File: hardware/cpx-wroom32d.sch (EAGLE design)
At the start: 37 parts, among them Q1 mmbt2222, Q2 mmbt2222, U1 ESP32-WROOM-32D

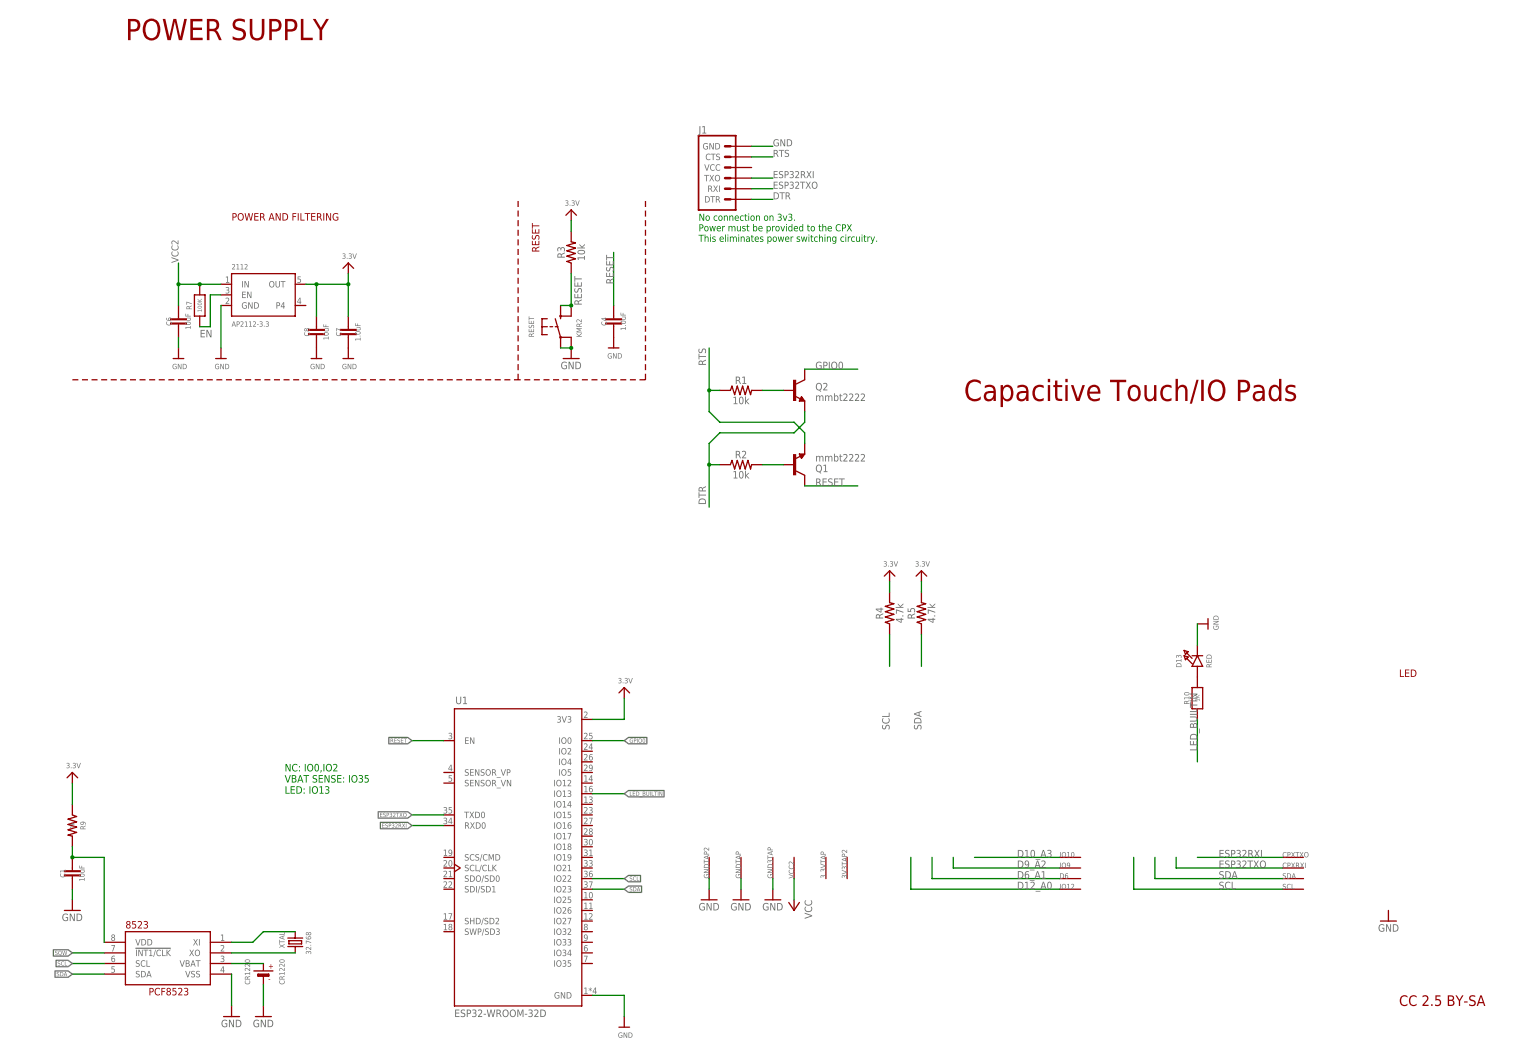
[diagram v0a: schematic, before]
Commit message: Looks goo.
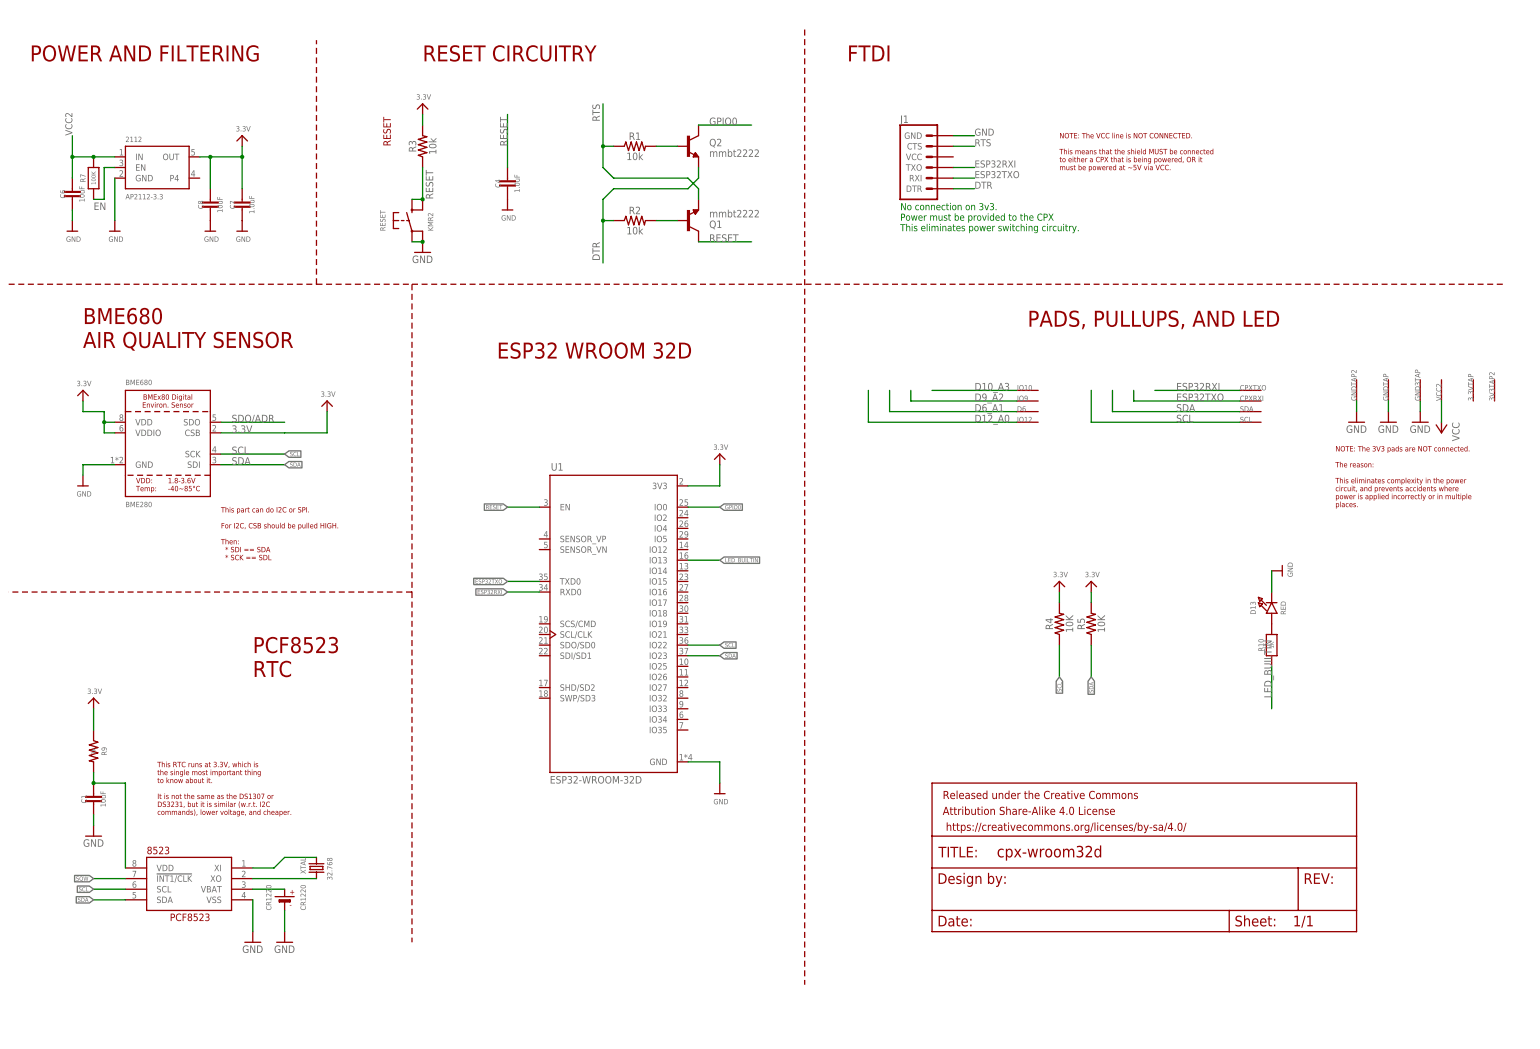
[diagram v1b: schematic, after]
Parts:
- added BME680: BME280, microbuilder:BME280
- added FRAME1: FRAME-LETTERNO_PACKAGE, SparkFun-Aesthetics:FRAME-LETTERNO_PACKAGE
- R4, R5: value 4.7k -> 10K
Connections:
- new net SDO/ADR: BME680.SDO
- net 3.3V: now also BME680.CSB, BME680.VDD, BME680.VDDIO
- net GND: now also BME680.GND
- net SCL: now also BME680.SCK
- net SDA: now also BME680.SDI
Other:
- note added: "BME680 AIR QUALITY SENSOR"
- note added: "ESP32 WROOM 32D"
- note added: "FTDI"
- note added: "NOTE: The 3V3 pads are NOT connected. The reason: This eliminates complexity in the power circuit, and prevents accidents where power is applied incorrectly or in multiple places."
- note added: "NOTE: The VCC line is NOT CONNECTED. This means that the shield MUST be connected to either a CPX that is being powered, OR it must be powered at ~5V via VCC."
- note added: "PADS, PULLUPS, AND LED"
- note added: "PCF8523 RTC"
- note added: "RESET CIRCUITRY"
- note added: "This RTC runs at 3.3V, which is the single most important thing to know about it. It is not the same as the DS1307 or DS3231, but it is similar (w.r.t. I2C commands), lower voltage, and cheaper."
- note added: "This part can do I2C or SPI. For I2C, CSB should be pulled HIGH. Then: * SDI == SDA * SCK == SDL"
- note removed: "CC 2.5 BY-SA"
- note removed: "Capacitive Touch/IO Pads"
- note removed: "LED"
- note removed: "NC: IO0,IO2 VBAT SENSE: IO35 LED: IO13"
- note removed: "POWER SUPPLY"
- moved on the sheet: 2112, 3.3VTAP, 3V3TAP2, 8523, C1, C4, C6, C7, C8, CPXRXI, CPXTXO, CR1220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
